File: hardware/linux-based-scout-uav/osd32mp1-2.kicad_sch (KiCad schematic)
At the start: 9 parts, among them J3 TC2050-IDC-NL, U1 OSD32MP157C-512M-IAA, Y1 ABS05-32.768KHZ-7-T

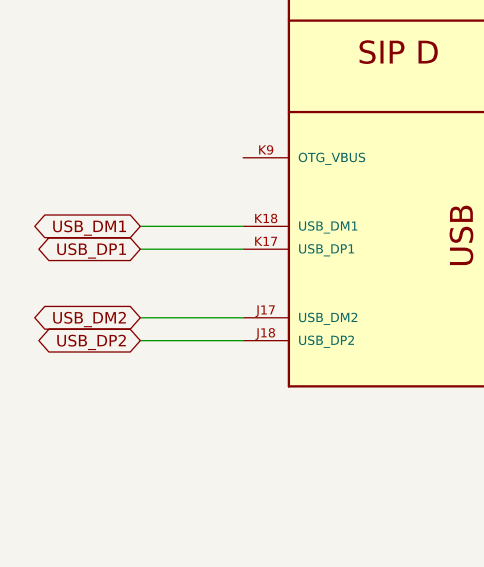
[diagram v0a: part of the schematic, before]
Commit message: Schematic and board update
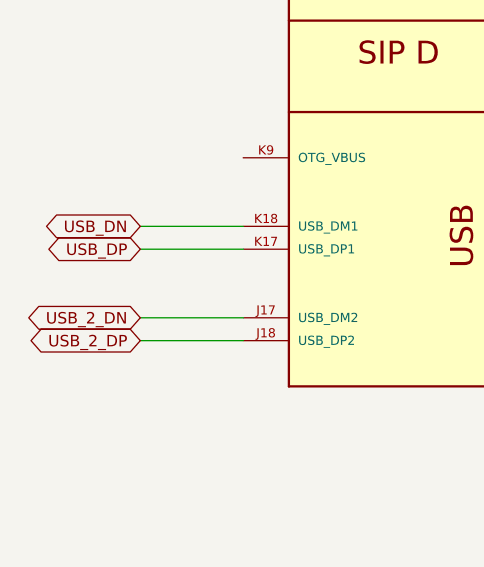
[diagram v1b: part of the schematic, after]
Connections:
- net USB_DM1 renamed USB_DN
- net USB_DM2 renamed USB_2_DN
- net USB_DP1 renamed USB_DP
- net USB_DP2 renamed USB_2_DP
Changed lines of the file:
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@@
 		)
 	)
-	(global_label "USB_DP2"
+	(global_label "USB_2_DP"
 		(shape bidirectional)
 		(at 38.1 163.83 180)
@@
 		)
 		(property "Intersheetrefs" "${INTERSHEET_REFS}"
-			(at 25.4764 163.83 0)
-			(effects
-				(font
-					(size 1.27 1.27)
-				)
-				(justify right)
-				(hide yes)
-			)
-		)
-	)
-	(global_label "USB_DM2"
+			(at 24.5088 163.83 0)
+			(effects
+				(font
+					(size 1.27 1.27)
+				)
+				(justify right)
+				(hide yes)
+			)
+		)
+	)
+	(global_label "USB_2_DN"
 		(shape bidirectional)
 		(at 38.1 161.29 180)
@@
 		)
 		(property "Intersheetrefs" "${INTERSHEET_REFS}"
-			(at 25.295 161.29 0)
+			(at 24.4483 161.29 0)
 			(effects
 				(font
@@
 		)
 	)
-	(global_label "USB_DM1"
+	(global_label "USB_DN"
 		(shape bidirectional)
 		(at 38.1 151.13 180)
@@
 		)
 		(property "Intersheetrefs" "${INTERSHEET_REFS}"
-			(at 25.295 151.13 0)
+			(at 26.6254 151.13 0)
 			(effects
 				(font
@@
 		)
 	)
-	(global_label "USB_DP1"
+	(global_label "USB_DP"
 		(shape bidirectional)
 		(at 38.1 153.67 180)
@@
 		)
 		(property "Intersheetrefs" "${INTERSHEET_REFS}"
-			(at 25.4764 153.67 0)
-			(effects
-				(font
+			(at 26.6859 153.67 0)
+			(effects
+				(font
